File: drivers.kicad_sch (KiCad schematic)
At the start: 16 parts, among them J1 Conn_01x04_Pin, U2 TMC2209-LA

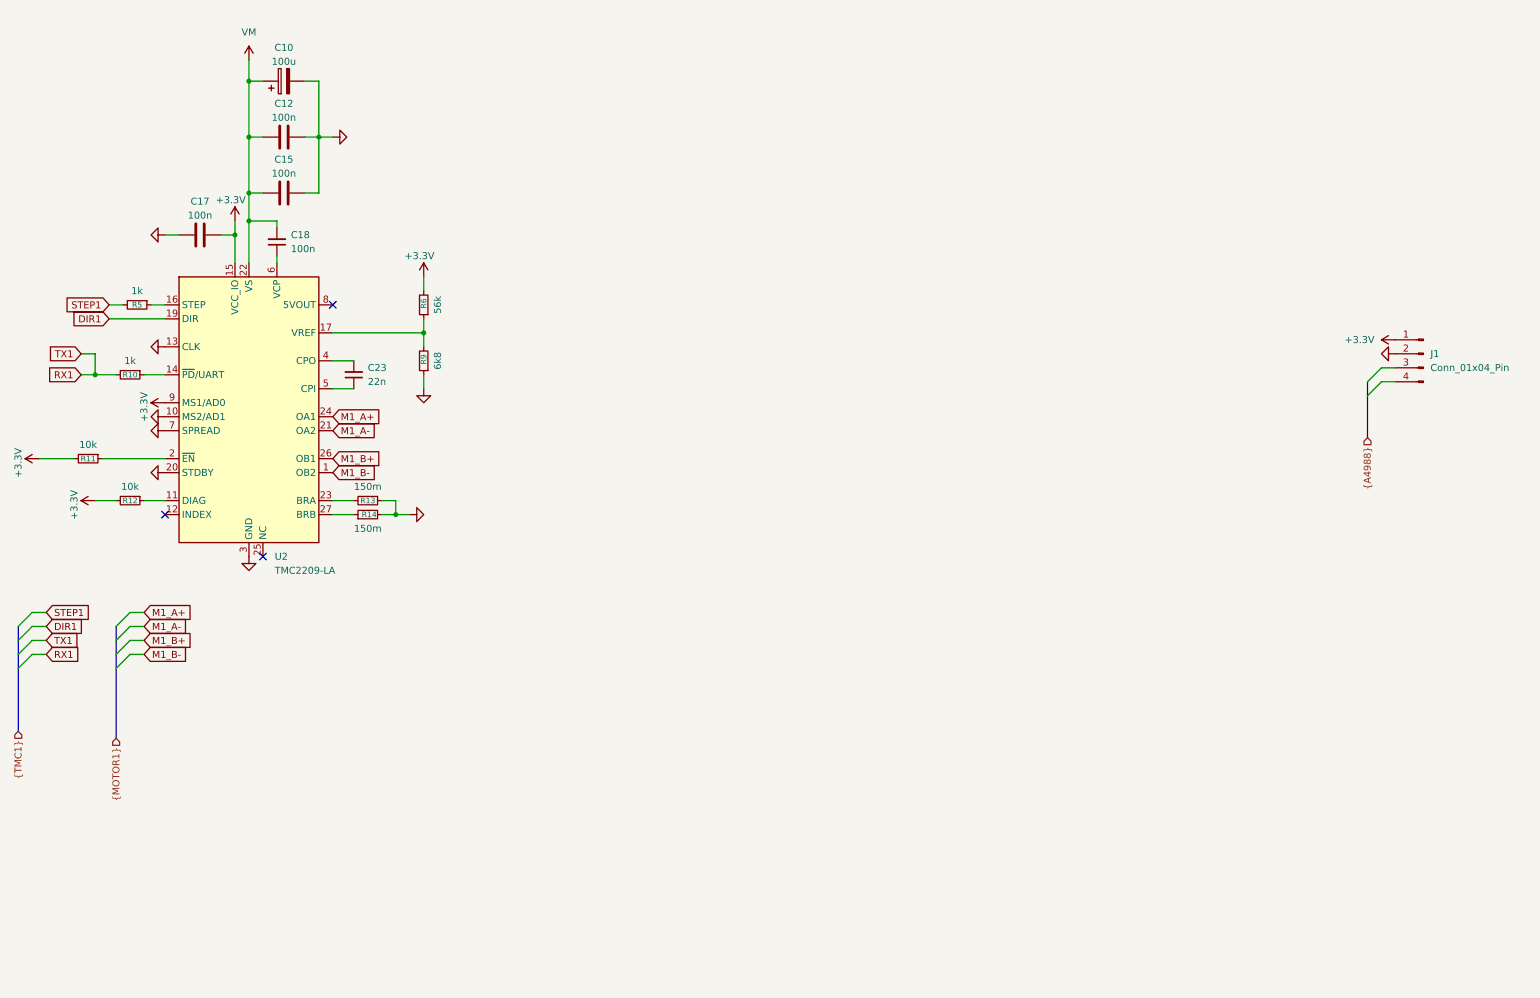
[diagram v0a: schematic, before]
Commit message: PCB schematic design
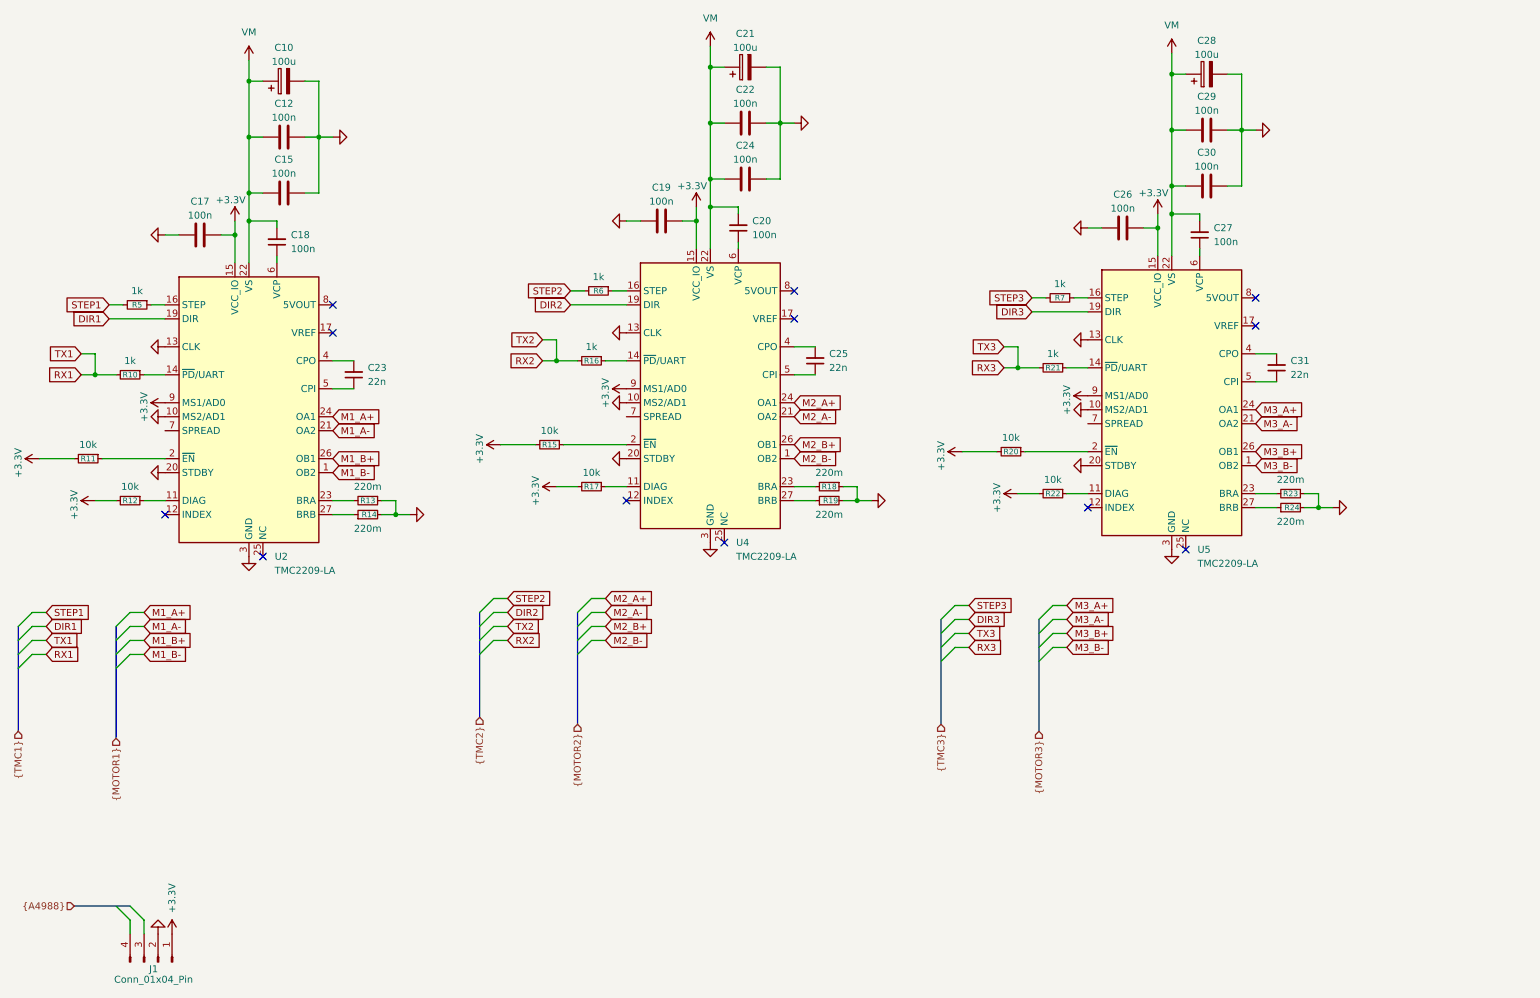
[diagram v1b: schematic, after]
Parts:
- removed R9: 6k8, symbol Device:R_Small
- added C19, C22, C24, C26, C29, C30: 100n, symbol Device:C
- added C20, C27: 100n, symbol Device:C_Small
- added C21, C28: 100u, symbol Device:C_Polarized
- added C25, C31: 22n, symbol Device:C_Small
- added R15, R17, R20, R22: 10k, symbol Device:R_Small
- added R16, R21, R7: 1k, symbol Device:R_Small
- added R18, R19, R23, R24: 220m, symbol Device:R_Small
- added U4, U5: TMC2209-LA, Package_DFN_QFN:VQFN-28-1EP_5x5mm_P0.5mm_EP3.7x3.7mm, symbol Driver_Motor:TMC2209-LA
- R13, R14: value 150m -> 220m
- R6: value 56k -> 1k
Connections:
- net +3.3V: now also C19.2, C26.2, R15.2, R17.2, R20.2, R22.2, U4.15 (VCC_IO), U4.9 (MS1/AD0), U5.15 (VCC_IO), U5.9 (MS1/AD0); no longer R6.2
- net GND: now also C19.1, C21.2, C22.2, C24.2, C26.1, C28.2, C29.2, C30.2, R18.1, R19.2, R23.1, R24.2, U4.10 (MS2/AD1), U4.13 (CLK), U4.18 (GND), U4.20 (STDBY), U4.29 (GND), U4.3 (GND), U5.10 (MS2/AD1), U5.13 (CLK), U5.18 (GND), U5.20 (STDBY), U5.29 (GND), U5.3 (GND); no longer U2.7 (SPREAD)
- net VM: now also C20.2, C21.1, C22.1, C24.1, C27.2, C28.1, C29.1, C30.1, U4.22 (VS), U4.28 (VS), U5.22 (VS), U5.28 (VS)
- net at R6.1: now also U4.16 (STEP); no longer U2.17 (VREF)
- new net: C31.1, U5.5 (CPI)
- new net: C31.2, U5.4 (CPO)
- new net: R19.1, U4.27 (BRB)
- new net: R20.1, U5.2 (~{EN})
- new net: R22.1, U5.11 (DIAG)
- new net: R23.2, U5.23 (BRA)
- new net: R16.1, U4.14 (~{PD}/UART)
- new net: R21.1, U5.14 (~{PD}/UART)
- new net: R24.1, U5.27 (BRB)
- new net: R7.1, U5.16 (STEP)
- new net: C27.1, U5.6 (VCP)
- new net: C25.1, U4.5 (CPI)
- new net: C25.2, U4.4 (CPO)
- new net: R17.1, U4.11 (DIAG)
- new net: R15.1, U4.2 (~{EN})
- new net: R18.2, U4.23 (BRA)
- new net: C20.1, U4.6 (VCP)
- new net DIR2: U4.19 (DIR)
- new net DIR3: U5.19 (DIR)
- new net M2_A+: U4.24 (OA1)
- new net M2_A-: U4.21 (OA2)
- new net M2_B+: U4.26 (OB1)
- new net M2_B-: U4.1 (OB2)
- new net M3_A+: U5.24 (OA1)
- new net M3_A-: U5.21 (OA2)
- new net M3_B+: U5.26 (OB1)
- new net M3_B-: U5.1 (OB2)
- new net RX2: R16.2
- new net RX3: R21.2
- new net STEP2: R6.2
- new net STEP3: R7.2
- no-connect marks 3 -> 12
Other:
- moved on the sheet: J1
